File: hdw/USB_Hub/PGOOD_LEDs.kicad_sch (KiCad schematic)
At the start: 12 parts

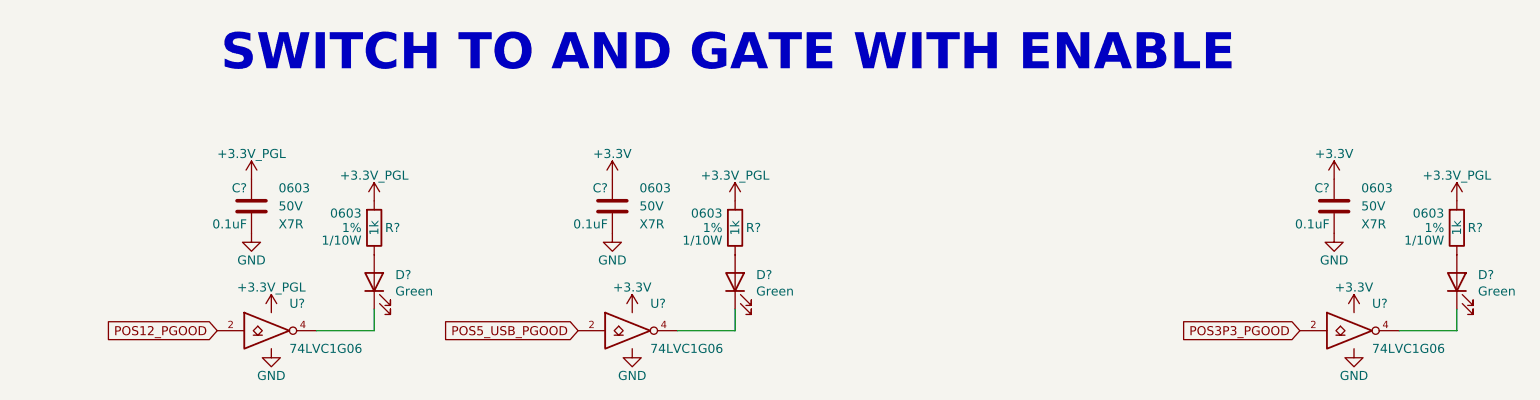
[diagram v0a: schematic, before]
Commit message: schematic progress
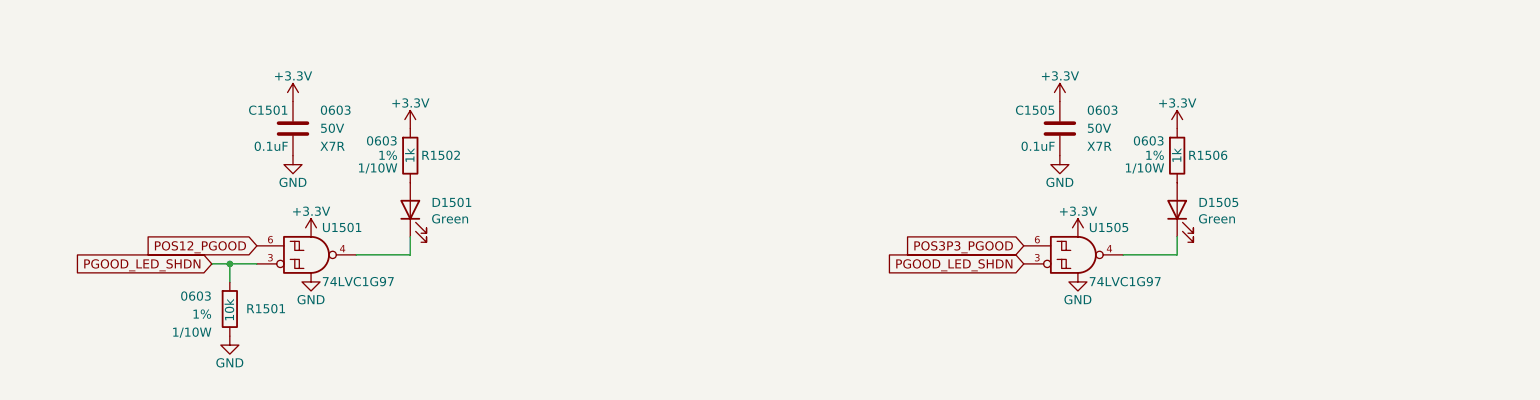
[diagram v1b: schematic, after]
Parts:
- removed C? (x3): 0.1uF, Capacitors_SMD:C_0603, symbol Custom_Library:C_Custom
- removed D? (x3): Green, LEDs:LED_0603, symbol Device:LED
- removed R? (x3): 1k, Resistors_SMD:R_0603, symbol Custom_Library:R_Custom
- removed U? (x3): 74LVC1G06, TO_SOT_Packages_SMD:SOT-353_SC-70-5, symbol Custom_Library:74LVC1G06_Power
- added C1501, C1505: 0.1uF, Capacitors_SMD:C_0603, symbol Custom_Library:C_Custom
- added D1501, D1505: Green, LEDs:LED_0603, symbol Device:LED
- added R1501: 10k, Resistors_SMD:R_0603, symbol Custom_Library:R_Custom
- added R1502, R1506: 1k, Resistors_SMD:R_0603, symbol Custom_Library:R_Custom
- added U1501, U1505: 74LVC1G97, Package_TO_SOT_SMD:SOT-363_SC-70-6, symbol Custom_Library:74LVC1G97_Power_NAND_INV
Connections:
- net +3.3V: now also C1501.1, C1505.1, R1502.1, R1506.1, U1501.1 (VCC), U1501.5 (VCC), U1505.1 (VCC), U1505.5 (VCC)
- net GND: now also C1501.2, C1505.2, R1501.2, U1501.2 (GND), U1505.2 (GND)
- net POS12_PGOOD: now also U1501.6
- net POS3P3_PGOOD: now also U1505.6
- new net: D1501.1 (K), U1501.4
- new net: D1501.2 (A), R1502.2
- new net: D1505.1 (K), U1505.4
- new net: D1505.2 (A), R1506.2
- new net PGOOD_LED_SHDN: R1501.1, U1501.3, U1505.3
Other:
- note removed: "SWITCH TO AND GATE WITH ENABLE"

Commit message: lots of schematic progress
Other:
- title: Analog Clock -> USB Hub
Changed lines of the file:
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@@
   (paper "A")
   (title_block
-    (title "Analog Clock")
-    (date "2020-08-15")
-    (rev "A")
+    (title "USB Hub")
+    (date "2023-08-18")
+    (rev "PRELIM")
     (company "Drew Maatman")
   )

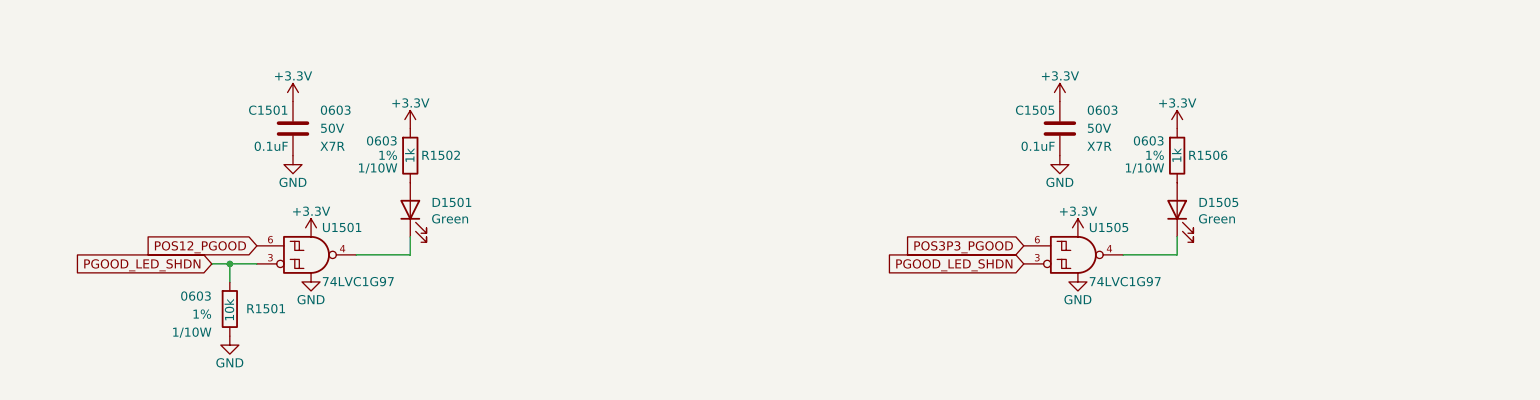
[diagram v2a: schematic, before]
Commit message: much more schematic progress
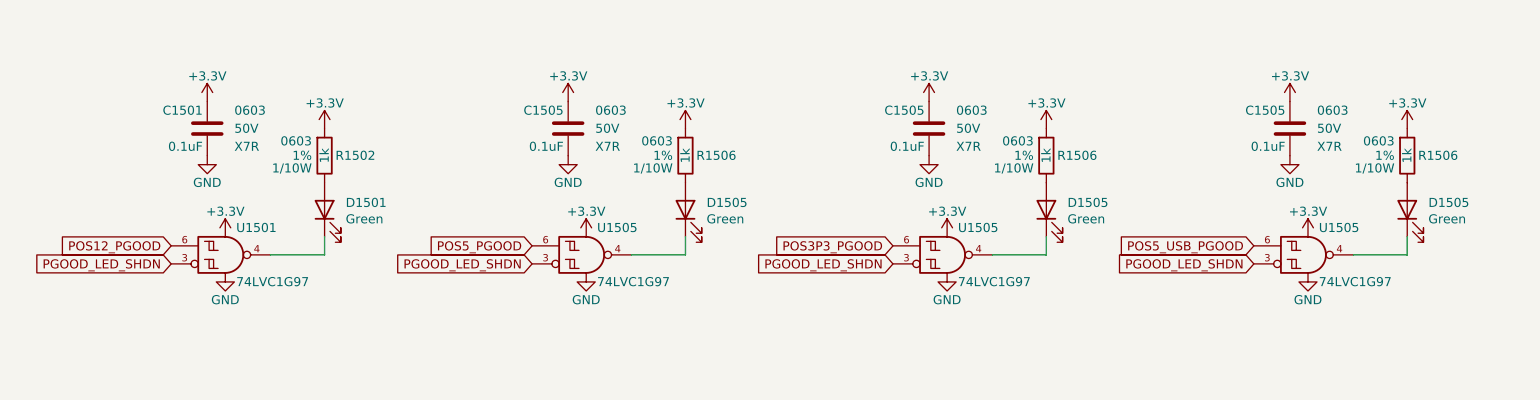
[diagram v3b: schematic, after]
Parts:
- removed R1501: 10k, Resistors_SMD:R_0603, symbol Custom_Library:R_Custom
- added C1505 (x2): 0.1uF, Capacitors_SMD:C_0603, symbol Custom_Library:C_Custom
- added D1505 (x2): Green, LEDs:LED_0603, symbol Device:LED
- added R1506 (x2): 1k, Resistors_SMD:R_0603, symbol Custom_Library:R_Custom
- added U1505 (x2): 74LVC1G97, Package_TO_SOT_SMD:SOT-363_SC-70-6, symbol Custom_Library:74LVC1G97_Power_NAND_INV
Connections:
- net +3.3V: now also C1505.1, C1505.1, R1506.1, R1506.1, U1505.1 (VCC), U1505.1 (VCC), U1505.5 (VCC), U1505.5 (VCC)
- net GND: now also C1505.2, C1505.2, U1505.2 (GND), U1505.2 (GND)
- net PGOOD_LED_SHDN: now also U1505.3, U1505.3
- new net: D1505.1 (K), U1505.4 (x2)
- new net: D1505.2 (A), R1506.2 (x2)
- new net POS5_PGOOD: U1505.6
- new net POS5_USB_PGOOD: U1505.6
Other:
- moved on the sheet: C1501, C1505, D1501, D1505, R1502, R1506, U1501, U1505
